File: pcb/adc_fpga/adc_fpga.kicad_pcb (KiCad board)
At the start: 4 copper layers, 85.5 x 54.5 mm, 49 parts, among them J1 RF_IN, J3 AUX I/O, J5 AUX I/O, Q1 BSS138, Q2 BSS138, U1 MAX4230AXK, U2 CMOD S7, U3 ADC14L020CIVY/NOPB, U4 TLV76133DCY

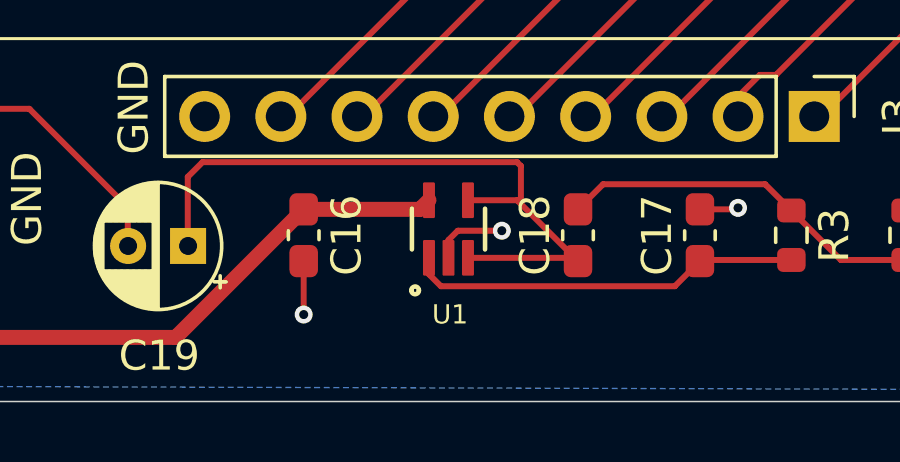
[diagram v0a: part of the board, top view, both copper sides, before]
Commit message: LCD kind of working
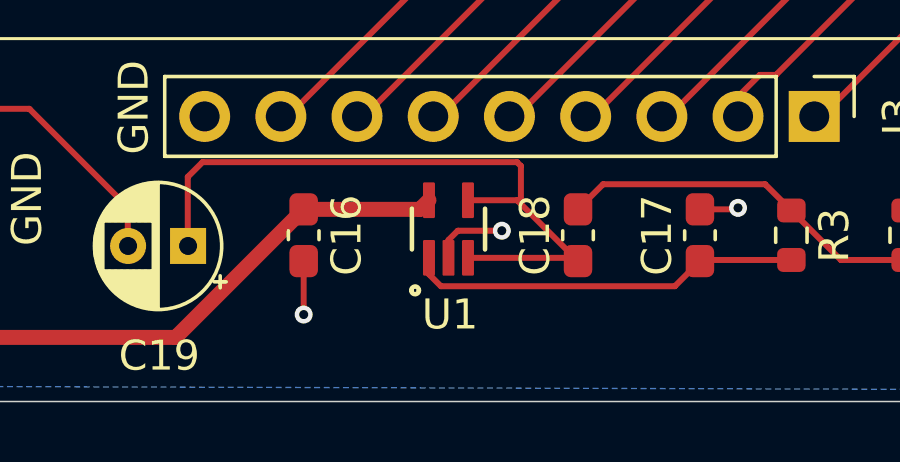
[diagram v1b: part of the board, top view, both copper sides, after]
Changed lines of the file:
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@@
 		(tags "resistor")
 		(property "Reference" "R6"
-			(at 0 -1.43 270)
+			(at 0 -1.43 -90)
 			(layer "F.SilkS")
 			(effects
@@
 		)
 		(property "Value" "10k"
-			(at 0 1.43 270)
+			(at 0 1.43 -90)
 			(layer "F.Fab")
 			(effects
@@
 		)
 		(fp_text user "${REFERENCE}"
-			(at 0 0 270)
+			(at 0 0 -90)
 			(layer "F.Fab")
 			(effects
@@
 		)
 		(fp_text user "${REFERENCE}"
-			(at 0 6.35 270)
+			(at 0 6.35 -90)
 			(layer "F.Fab")
 			(effects
@@
 		(tags "resistor")
 		(property "Reference" "R7"
-			(at 0 -1.43 270)
+			(at 0 -1.43 -90)
 			(layer "F.SilkS")
 			(effects
@@
 		)
 		(property "Value" "10k"
-			(at 0 1.43 270)
+			(at 0 1.43 -90)
 			(layer "F.Fab")
 			(effects
@@
 		)
 		(fp_text user "${REFERENCE}"
-			(at 0 0 270)
+			(at 0 0 -90)
 			(layer "F.Fab")
 			(effects
@@
 		(tags "resistor")
 		(property "Reference" "R8"
-			(at 0 -1.43 270)
+			(at 0 -1.43 -90)
 			(layer "F.SilkS")
 			(effects
@@
 		)
 		(property "Value" "10k"
-			(at 0 1.43 270)
+			(at 0 1.43 -90)
 			(layer "F.Fab")
 			(effects
@@
 		)
 		(fp_text user "${REFERENCE}"
-			(at 0 0 270)
+			(at 0 0 -90)
 			(layer "F.Fab")
 			(effects
@@
 		(tags "SOT TO_SOT_SMD")
 		(property "Reference" "Q1"
-			(at 0 -2.4 270)
+			(at 0 -2.4 -90)
 			(layer "F.SilkS")
 			(effects
@@
 		)
 		(property "Value" "BSS138"
-			(at 0 2.4 270)
+			(at 0 2.4 -90)
 			(layer "F.Fab")
 			(effects
@@
 		)
 		(fp_text user "${REFERENCE}"
-			(at 0 0 270)
+			(at 0 0 -90)
 			(layer "F.Fab")
 			(effects
@@
 		(tags "SOT TO_SOT_SMD")
 		(property "Reference" "Q2"
-			(at 0 -2.4 270)
+			(at 0 -2.4 -90)
 			(layer "F.SilkS")
 			(effects
@@
 		)
 		(property "Value" "BSS138"
-			(at 0 2.4 270)
+			(at 0 2.4 -90)
 			(layer "F.Fab")
 			(effects
@@
 		)
 		(fp_text user "${REFERENCE}"
-			(at 0 0 270)
+			(at 0 0 -90)
 			(layer "F.Fab")
 			(effects
@@
 			(effects
 				(font
-					(size 0.64 0.64)
+					(size 1 1)
 					(thickness 0.15)
 				)
@@
 		(tags "resistor")
 		(property "Reference" "R5"
-			(at 0 -1.43 270)
+			(at 0 -1.43 -90)
 			(layer "F.SilkS")
 			(effects
@@
 		)
 		(property "Value" "10k"
-			(at 0 1.43 270)
+			(at 0 1.43 -90)
 			(layer "F.Fab")
 			(effects
@@
 		)
 		(fp_text user "${REFERENCE}"
-			(at 0 0 270)
+			(at 0 0 -90)
 			(layer "F.Fab")
 			(effects
